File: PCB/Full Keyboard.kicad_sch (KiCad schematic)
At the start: 228 parts, among them J1 USB_C, J2 Keyswitch, K1 Keyswitch, M1 Keyswitch, P1 Keyswitch, Q1 Keyswitch, SW1 SW_Push, T1 Keyswitch, U1 STM32F072CBT6, U2 Keyswitch, U3 XC6206, U4 USBLC6-2SC6, X1 Keyswitch, Y1 Keyswitch

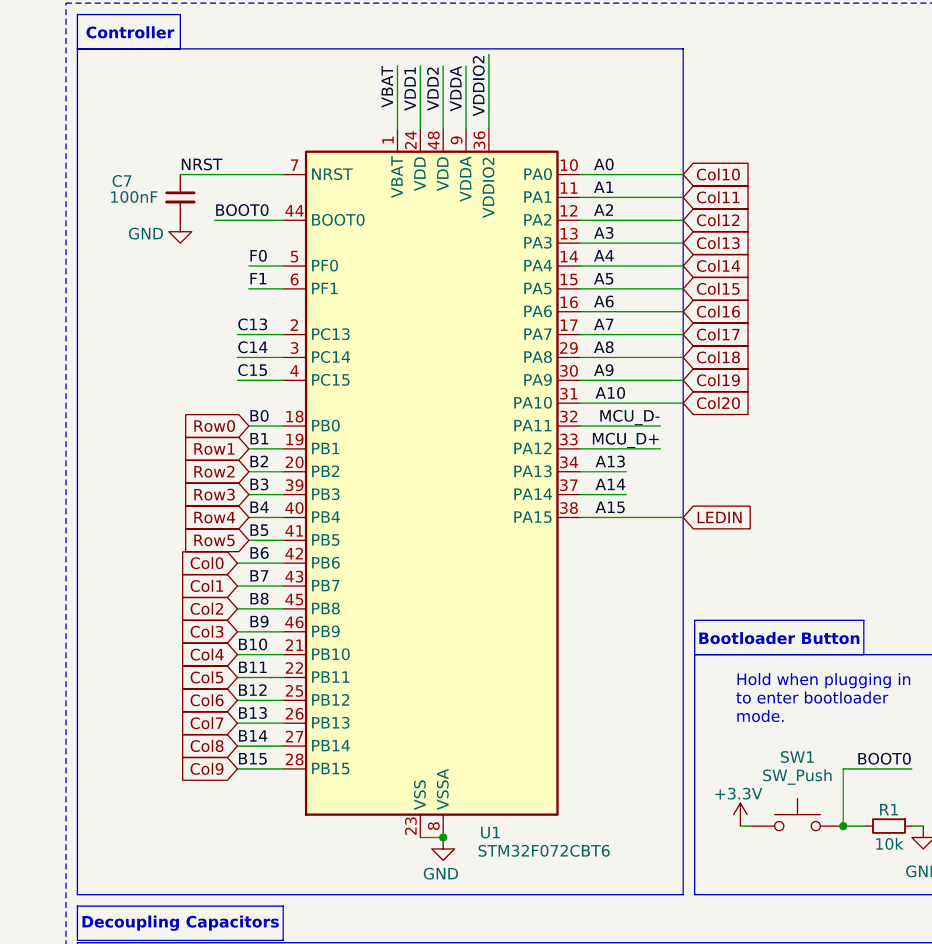
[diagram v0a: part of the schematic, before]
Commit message: update
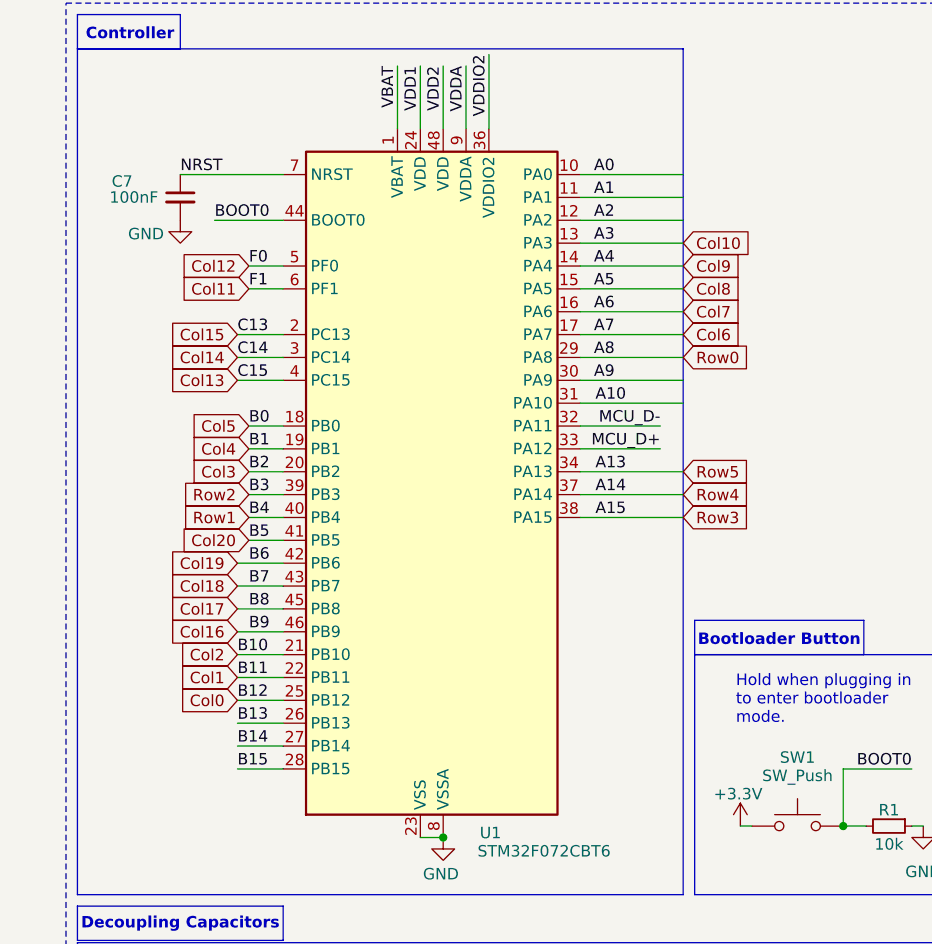
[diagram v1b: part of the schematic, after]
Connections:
- net A13 is gone; now on net Row5: U1.34 (PA13)
- net A14 is gone; now on net Row4: U1.37 (PA14)
- net C13 is gone; now on net Col15: U1.2 (PC13)
- net C14 is gone; now on net Col14: U1.3 (PC14)
- net C15 is gone; now on net Col13: U1.4 (PC15)
- net F0 is gone; now on net Col12: U1.5 (PF0)
- net F1 is gone; now on net Col11: U1.6 (PF1)
- net LEDIN is gone; now on net Row3: U1.38 (PA15)
- net Col0: now also U1.25 (PB12); no longer U1.42 (PB6)
- net Col1: now also U1.22 (PB11); no longer U1.43 (PB7)
- net Col10: now also U1.13 (PA3); no longer U1.10 (PA0)
- net Col11: no longer U1.11 (PA1)
- net Col12: no longer U1.12 (PA2)
- net Col13: no longer U1.13 (PA3)
- net Col14: no longer U1.14 (PA4)
- net Col15: no longer U1.15 (PA5)
- net Col16: now also U1.46 (PB9); no longer U1.16 (PA6)
- net Col17: now also U1.45 (PB8); no longer U1.17 (PA7)
- net Col18: now also U1.43 (PB7); no longer U1.29 (PA8)
- net Col19: now also U1.42 (PB6); no longer U1.30 (PA9)
- net Col2: now also U1.21 (PB10); no longer U1.45 (PB8)
- net Col20: now also U1.41 (PB5); no longer U1.31 (PA10)
- net Col3: now also U1.20 (PB2); no longer U1.46 (PB9)
- net Col4: now also U1.19 (PB1); no longer U1.21 (PB10)
- net Col5: now also U1.18 (PB0); no longer U1.22 (PB11)
- net Col6: now also U1.17 (PA7); no longer U1.25 (PB12)
- net Col7: now also U1.16 (PA6); no longer U1.26 (PB13)
- net Col8: now also U1.15 (PA5); no longer U1.27 (PB14)
- net Col9: now also U1.14 (PA4); no longer U1.28 (PB15)
- net Row0: now also U1.29 (PA8); no longer U1.18 (PB0)
- net Row1: now also U1.40 (PB4); no longer U1.19 (PB1)
- net Row2: now also U1.39 (PB3); no longer U1.20 (PB2)
- net Row3: no longer U1.39 (PB3)
- net Row4: no longer U1.40 (PB4)
- net Row5: no longer U1.41 (PB5)
- new net A0: U1.10 (PA0)
- new net A1: U1.11 (PA1)
- new net A10: U1.31 (PA10)
- new net A2: U1.12 (PA2)
- new net A9: U1.30 (PA9)
- new net B13: U1.26 (PB13)
- new net B14: U1.27 (PB14)
- new net B15: U1.28 (PB15)
